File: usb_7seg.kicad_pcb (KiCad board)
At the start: 2 copper layers, 72 x 47 mm, 7 parts, among them U1 SeeeduinoXIAO, U2 7segment_led, U3 TM1637

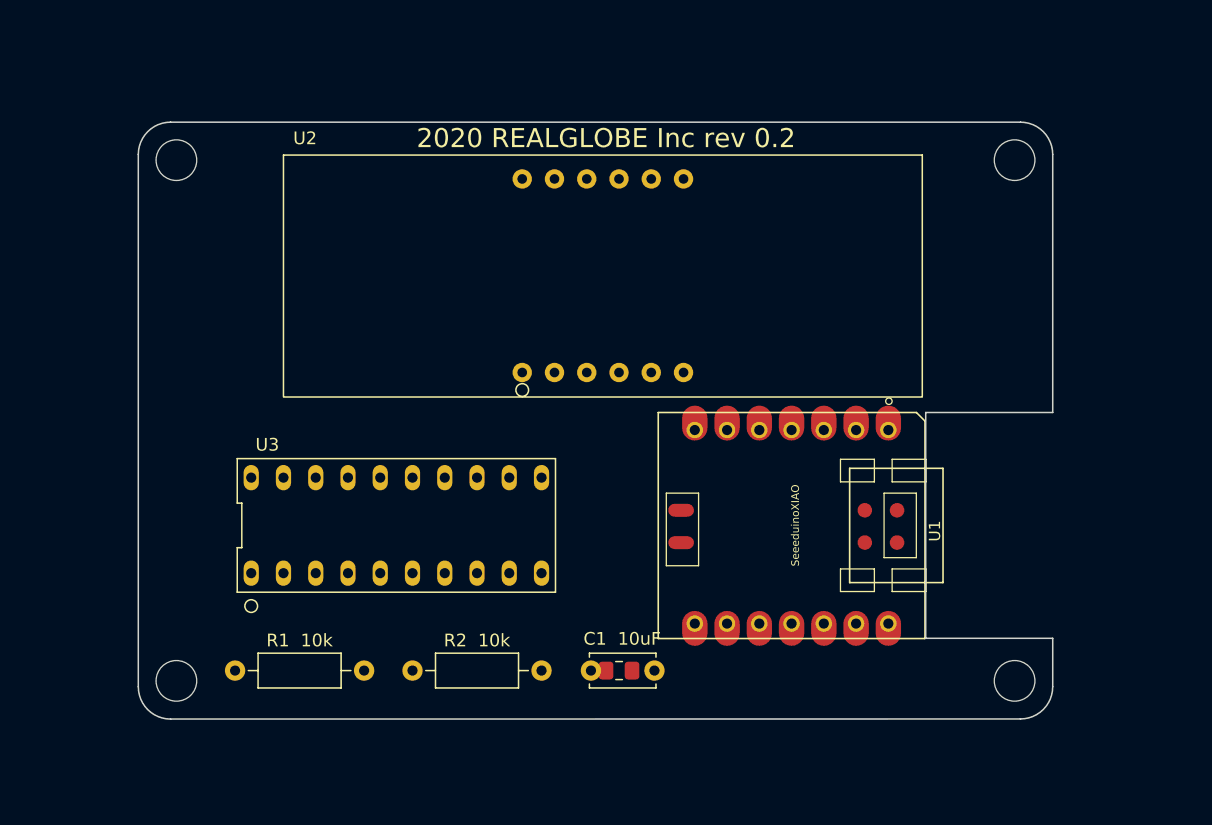
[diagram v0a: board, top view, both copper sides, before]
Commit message: とりあえず配線完了 DRC ok
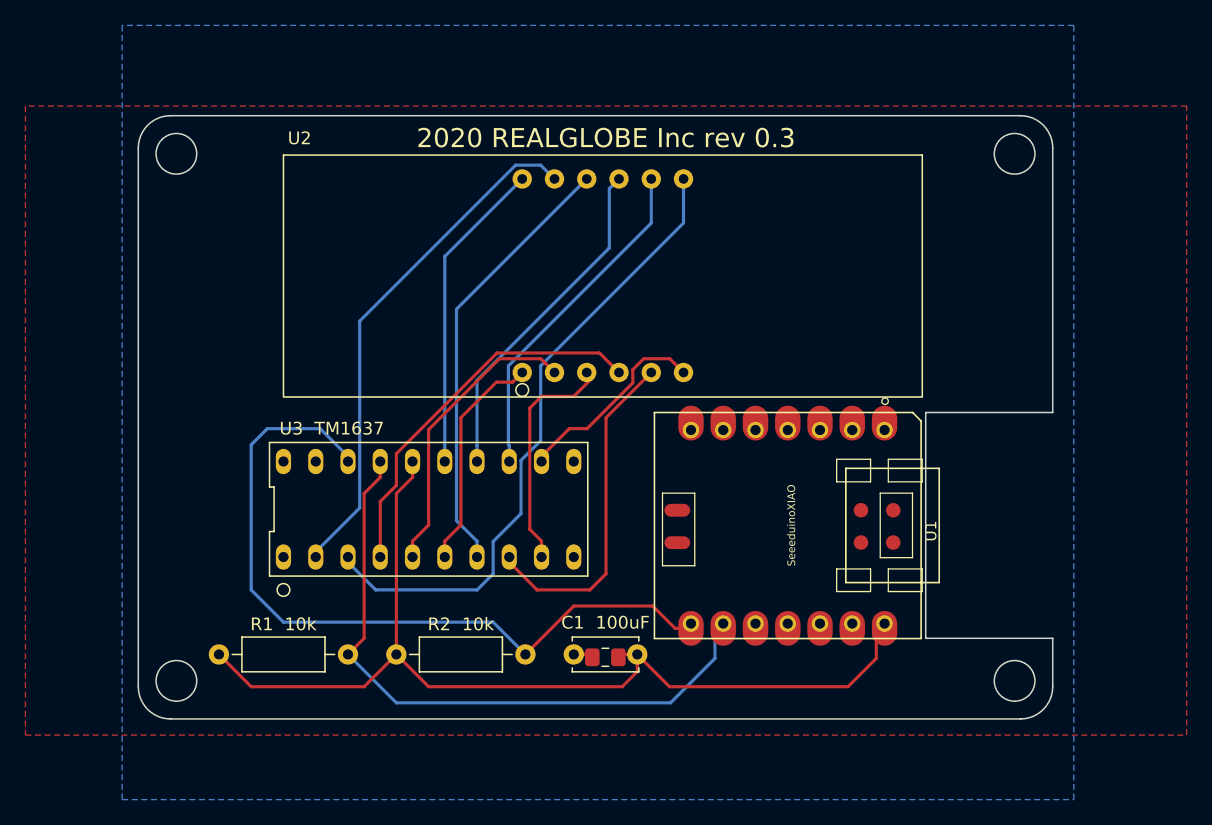
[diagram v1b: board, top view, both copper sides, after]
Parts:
- removed C1  10uF: 10uF, Capacitor_THT:C_Disc_D5.0mm_W2.5mm_P5.00mm
- removed U3: TM1637, kicad_mylib:TM1630
- added C1  100uF: 10uF, Capacitor_THT:C_Disc_D5.0mm_W2.5mm_P5.00mm, F.Cu at (34.3, -5.08)
- added U3  TM1637: TM1637, kicad_mylib:TM1630, F.Cu at (10.2, -11.4)
- added ~: akizuki_C_plate_lower_right, kicad_mylib:akizuki_C_plate_lower_right, F.Cu at (0.00, 0.00)
- moved R1  10k 1.80 mm to (6.35, -5.08)
- moved R2  10k 1.80 mm to (20.3, -5.08)
- moved ~ 1.50 mm to (36.8, -4.85)
- moved U1 0.30 mm to (40.6, -24.1)
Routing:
- net +5V: track 0.00 -> 79.0 mm
- net Net-(R2-Pad2): track 0.00 -> 59.9 mm
- net Net-(R1-Pad2): track 0.00 -> 51.2 mm
- net Net-(U2-Pad7): track 0.00 -> 50.6 mm
- net Net-(U2-Pad11): track 0.00 -> 40.9 mm
- net Net-(U2-Pad10): track 0.00 -> 34.7 mm
- net Net-(U2-Pad4): track 0.00 -> 30.1 mm
- net Net-(U2-Pad8): track 0.00 -> 26.9 mm
- net Net-(U2-Pad9): track 0.00 -> 26.9 mm
- net Net-(U2-Pad5): track 0.00 -> 26.8 mm
- net Net-(U2-Pad12): track 0.00 -> 24.8 mm
- net Net-(U2-Pad2): track 0.00 -> 23.2 mm
- net Net-(U2-Pad3): track 0.00 -> 18.5 mm
- net Net-(U2-Pad1): track 0.00 -> 17.8 mm
- net Net-(U2-Pad6): track 0.00 -> 15.8 mm
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- added copper zone on B.Cu, net GND
- added copper zone on F.Cu, net GND
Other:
- board size 72 x 47 mm -> 72 x 47.5 mm
- board text added: "2020 REALGLOBE Inc rev 0.3"
- board text removed: "2020 REALGLOBE Inc rev 0.2"
